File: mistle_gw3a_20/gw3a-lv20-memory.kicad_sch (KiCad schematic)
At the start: 9 parts, among them U13 MT48LC16M16A2TG, U6 W25Q128JVS

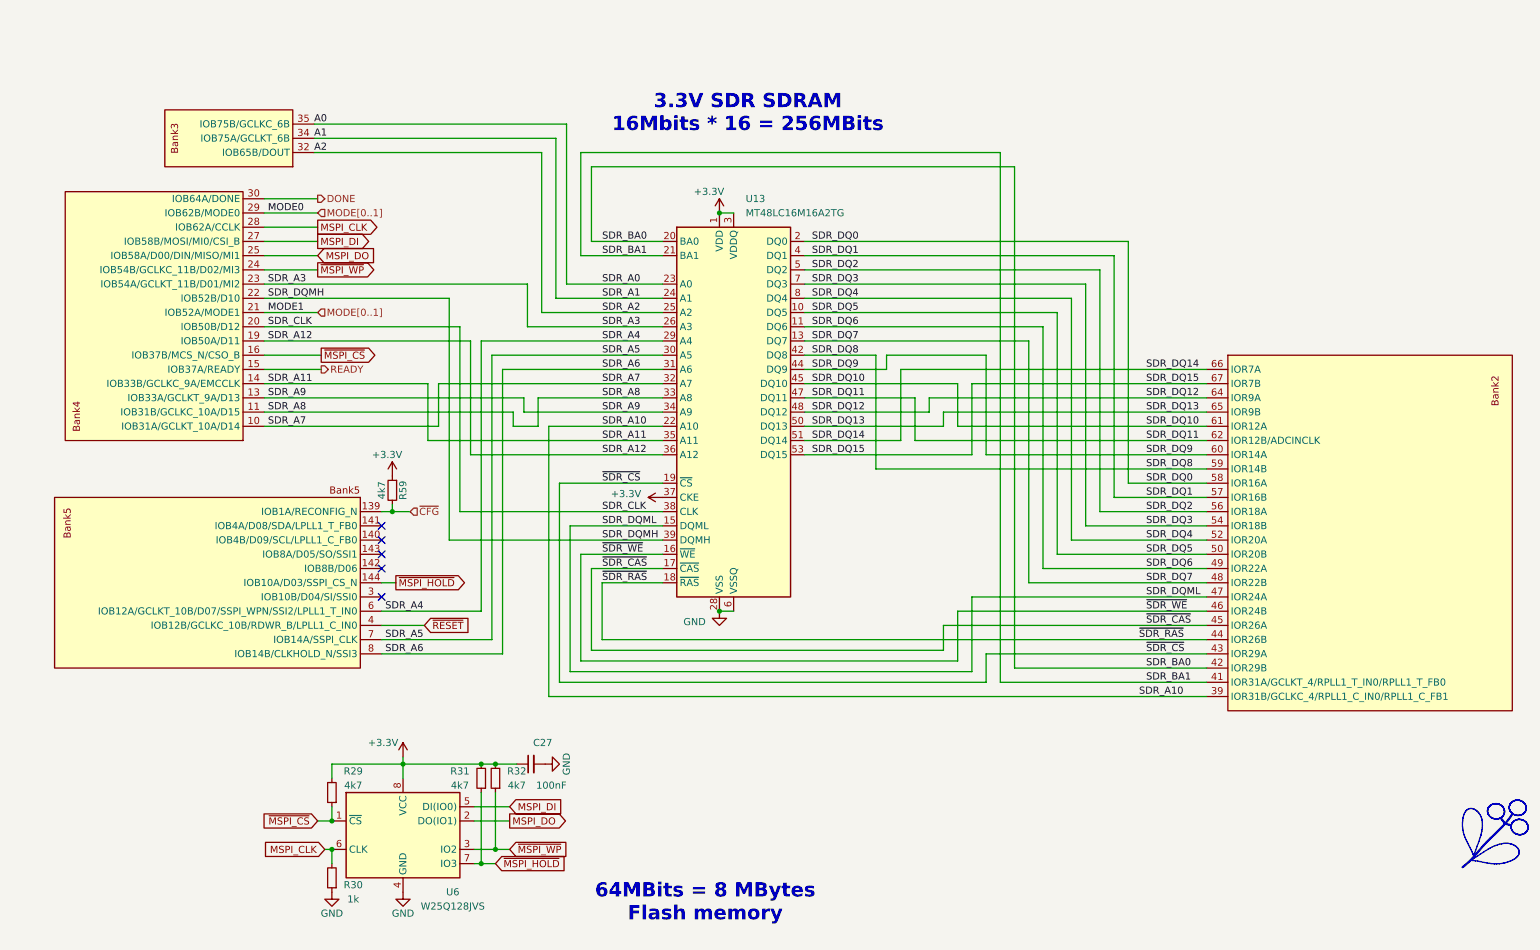
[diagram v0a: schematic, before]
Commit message: Update gw3a dev board
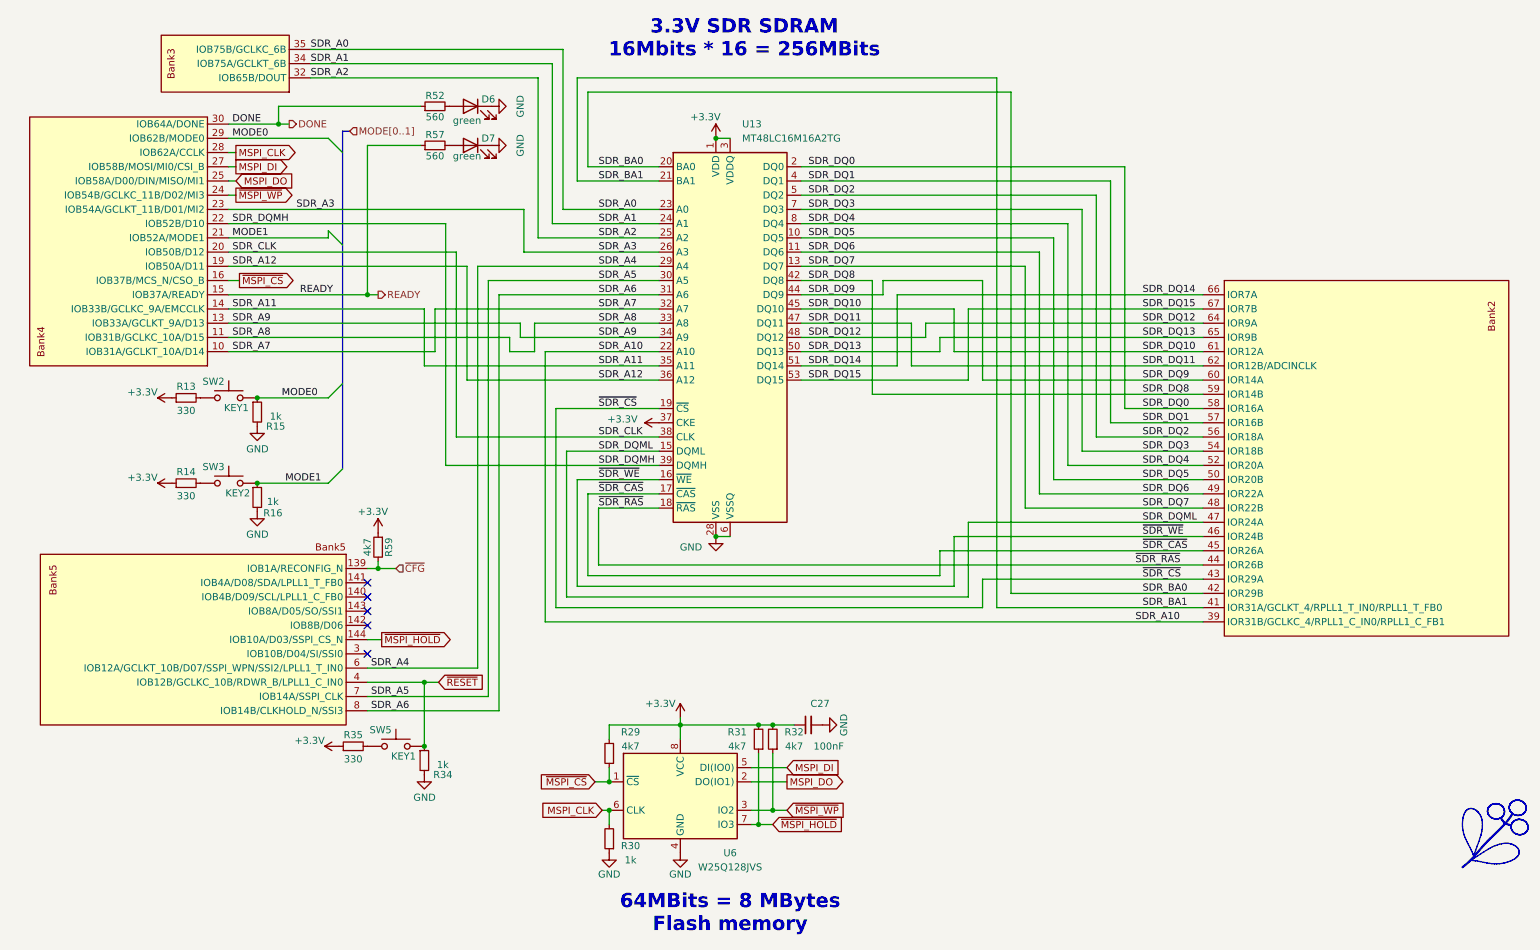
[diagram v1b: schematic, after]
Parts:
- added D6, D7: green, LED_SMD:LED_0805_2012Metric, symbol Device:LED
- added R13, R14, R35: 330, Resistor_SMD:R_0402_1005Metric, symbol Device:R_Small
- added R15, R16, R34: 1k, Resistor_SMD:R_0402_1005Metric, symbol Device:R_Small
- added R52, R57: 560, Resistor_SMD:R_0402_1005Metric, symbol Device:R_Small
- added SW2, SW5: KEY1, Button_Switch_SMD:SW_SPST_TL3342, symbol Switch:SW_Push
- added SW3: KEY2, Button_Switch_SMD:SW_SPST_TL3342, symbol Switch:SW_Push
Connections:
- net +3.3V: now also R13.1, R14.1, R35.1
- net DONE: now also R52.1
- net GND: now also D6.1 (K), D7.1 (K), R15.2, R16.2, R34.2
- net MODE[0..1]: no longer U7.21 (IOB52A/MODE1), U7.29 (IOB62B/MODE0)
- net READY: now also R57.1
- net ~{RESET}: now also R34.1, SW5.2
- net A0 renamed SDR_A0
- net A1 renamed SDR_A1
- net A2 renamed SDR_A2
- new net: R13.2, SW2.1
- new net: D6.2 (A), R52.2
- new net: D7.2 (A), R57.2
- new net: R35.2, SW5.1
- new net: R14.2, SW3.1
- new net MODE0: R15.1, SW2.2, U7.29 (IOB62B/MODE0)
- new net MODE1: R16.1, SW3.2, U7.21 (IOB52A/MODE1)
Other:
- moved on the sheet: C27, R29, R30, R31, R32, R59, U13, U6
